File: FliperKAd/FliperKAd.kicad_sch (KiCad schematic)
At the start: 29 parts, among them J1 Conn_01x02, J2 Conn_ST_STDC14, J3 Conn_01x02, J5 Conn_01x02, Q1 NMOS, U1 STM32G431KBTx, U3 MCP1640x-xMC

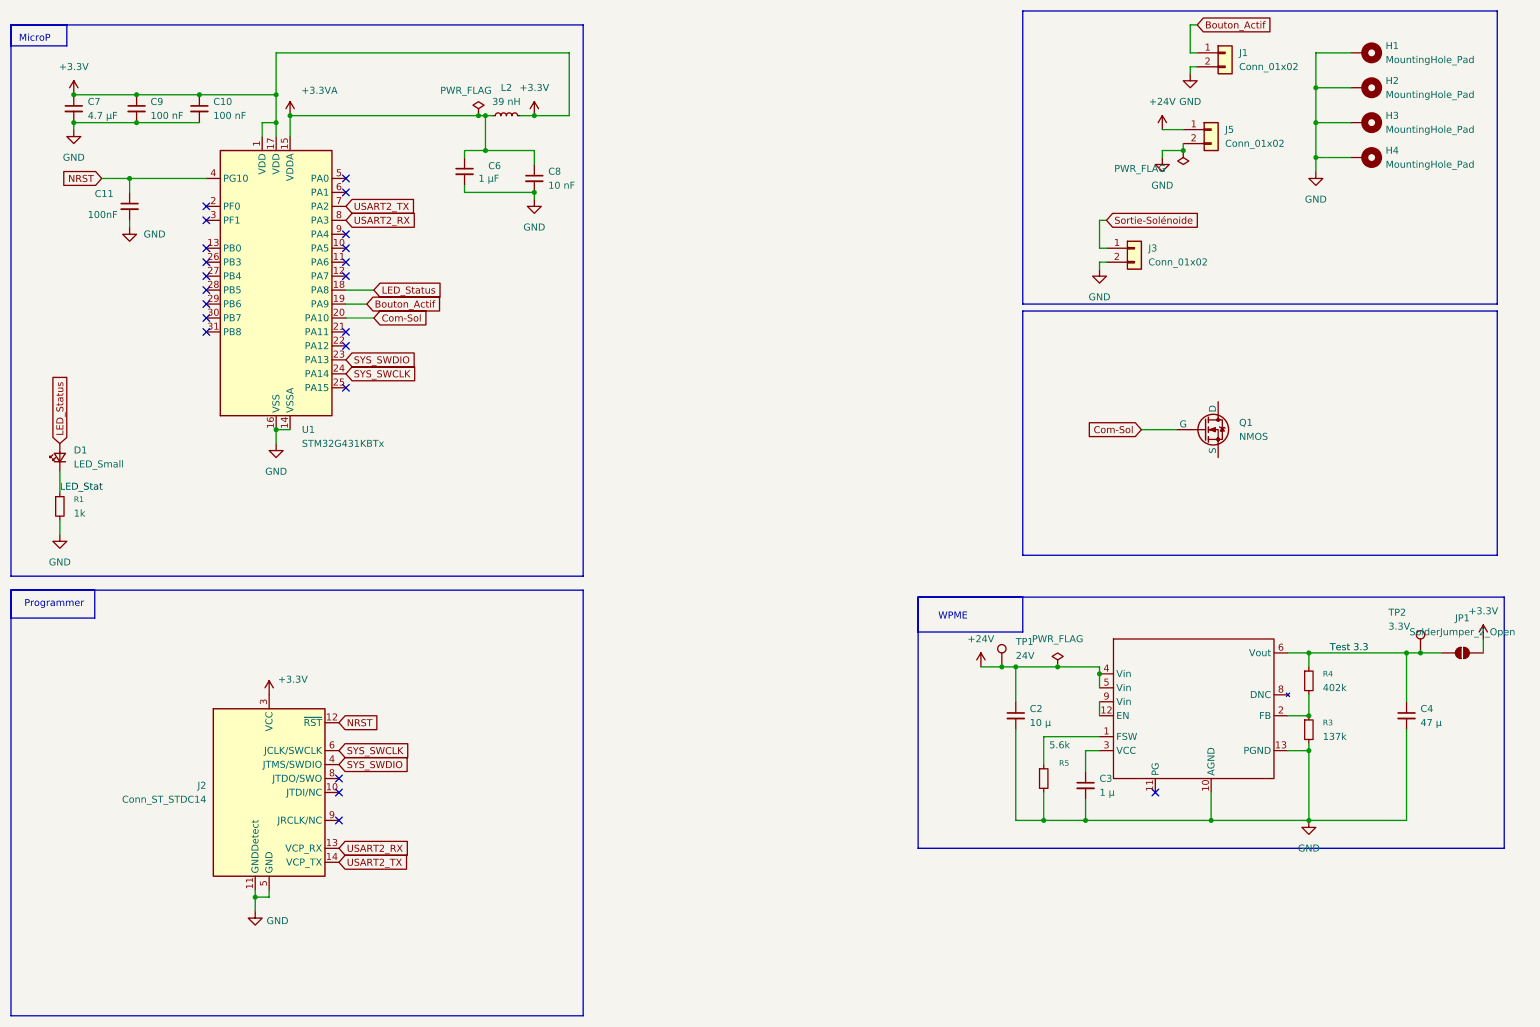
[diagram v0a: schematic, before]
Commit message: just in time
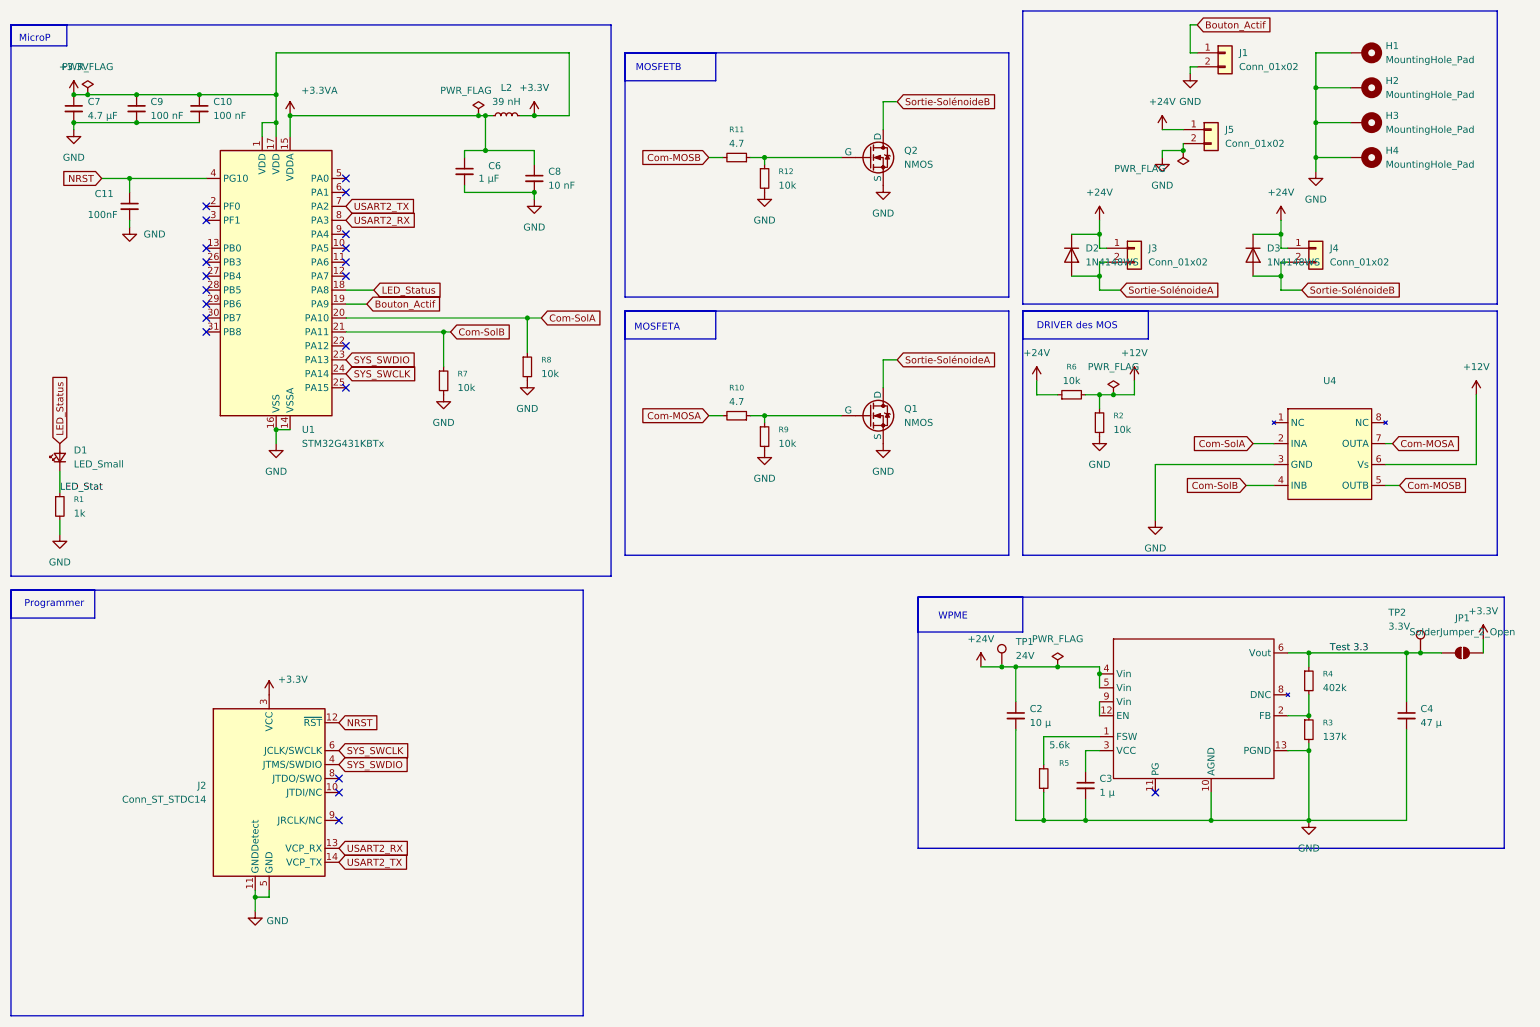
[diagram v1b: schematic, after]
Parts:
- added D2, D3: 1N4148WS, Diode_SMD:D_SOD-323, symbol Diode:1N4148WS
- added J4: Conn_01x02, Connector_JST:JST_XH_B2B-XH-A_1x02_P2.50mm_Vertical, symbol Connector_Generic:Conn_01x02
- added Q2: NMOS, Package_TO_SOT_SMD:TO-263-3_TabPin4, symbol Simulation_SPICE:NMOS
- added R10, R11: 4.7, Resistor_SMD:R_0603_1608Metric, symbol Device:R_Small
- added R12, R2, R6, R7, R8, R9: 10k, Resistor_SMD:R_0603_1608Metric, symbol Device:R_Small
- added U4: ~, Perso:MIC4426, symbol Lib:MIC4426
- Q1: footprint (none) -> Package_TO_SOT_SMD:TO-263-3_TabPin4
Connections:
- net Sortie-Solénoide is gone; now on net +24V: J3.1 (Pin_1)
- net +24V: now also D2.1 (K), D3.1 (K), J4.1 (Pin_1), R6.1
- net GND: now also Q1.3 (S), Q2.3 (S), R12.2, R2.2, R7.2, R8.2, R9.2, U4.3 (GND); no longer J3.2 (Pin_2)
- net Sortie-SolénoideA: now reaches Q1.1 (D)
- net Sortie-SolénoideA: now also J3.2 (Pin_2), D2.2 (A)
- net Com-SolB: now reaches U1.21 (PA11)
- net Com-SolB: now also R7.1, U4.4 (INB)
- net Com-Sol: no longer names the net of Q1.2 (G)
- net Com-Sol: now also R10.1, R9.1; no longer U1.20 (PA10)
- new net: Q2.2 (G), R11.1, R12.1
- new net +12V: R2.1, R6.2, U4.6 (Vs)
- new net Com-MOSA: R10.2, U4.7 (OUTA)
- new net Com-MOSB: R11.2, U4.5 (OUTB)
- new net Com-SolA: R8.1, U1.20 (PA10), U4.2 (INA)
- new net Sortie-SolénoideB: D3.2 (A), J4.2 (Pin_2), Q2.1 (D)
- no-connect marks 22 -> 21
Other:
- note added: "DRIVER des MOS"
- note added: "MOSFETA"
- note added: "MOSFETB"
- moved on the sheet: Q1
